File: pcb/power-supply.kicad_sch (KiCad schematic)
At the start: 6 parts, among them IC1 AP2112K-3.3TRG1

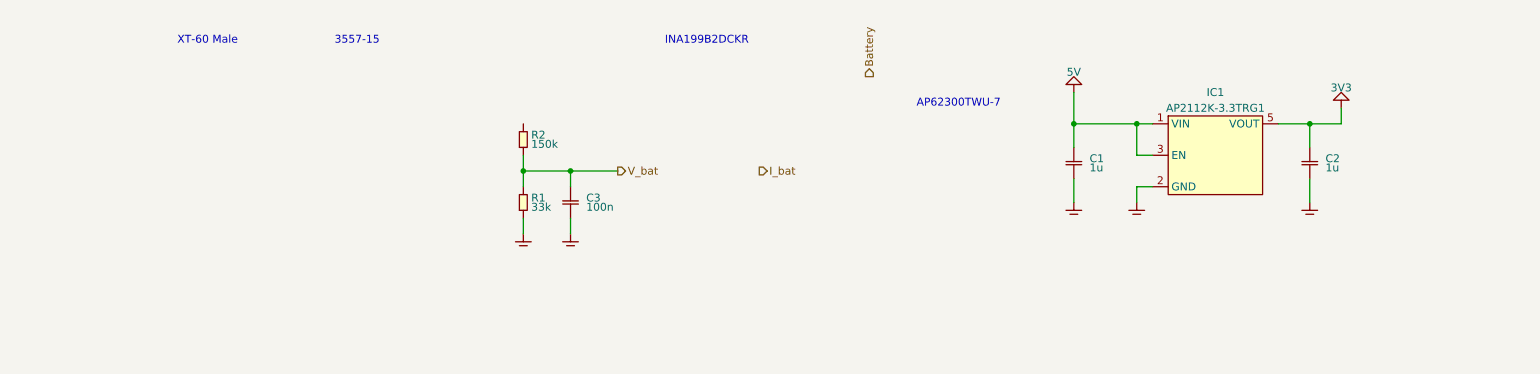
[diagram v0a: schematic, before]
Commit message: continued work on schematic
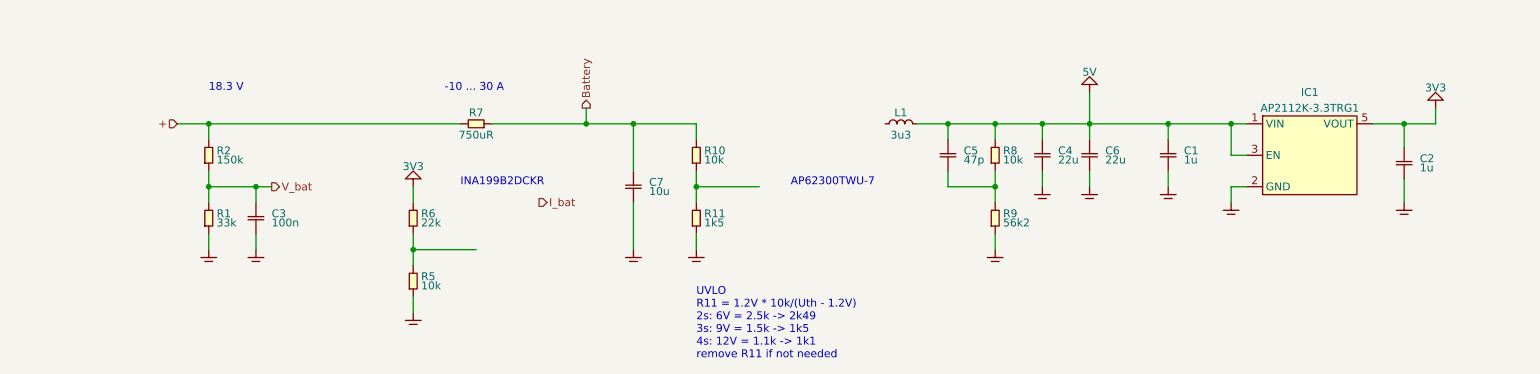
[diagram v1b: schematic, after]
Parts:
- added C4, C6: 22u, SMT:0603, symbol generic:C
- added C5: 47p, SMT:0603, symbol generic:C
- added C7: 10u, SMT:0603, symbol generic:C
- added L1: 3u3, symbol generic:L
- added R10, R5, R8: 10k, SMT:0603, symbol generic:R
- added R11: 1k5, SMT:0603, symbol generic:R
- added R6: 22k, SMT:0603, symbol generic:R
- added R7: 750uR, SMT:0603, symbol generic:R
- added R9: 56k2, SMT:0603, symbol generic:R
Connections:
- net 3V3: now also R6.2
- net Battery: now also C7.1, R10.2, R7.1
- net GND: now also C4.1, C4.2, C5.1, C6.1, C6.2, C7.2, L1.2, R11.1, R5.1, R8.2, R9.1
- net +: now reaches R2.2
- net +: now also R7.2
- new net: R10.1, R11.2
- new net: R5.2, R6.1
- new net: C5.2, R8.1, R9.2
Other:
- note added: "-10 ... 30 A"
- note added: "18.3 V"
- note added: "UVLO R11 = 1.2V * 10k/(Uth - 1.2V) 2s: 6V = 2.5k -> 2k49 3s: 9V = 1.5k -> 1k5 4s: 12V = 1.1k -> 1k1 remove R11 if not needed"
- note removed: "3557-15"
- note removed: "XT-60 Male"
- moved on the sheet: C1, C2, C3, IC1, R1, R2

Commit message: schematic mostly done
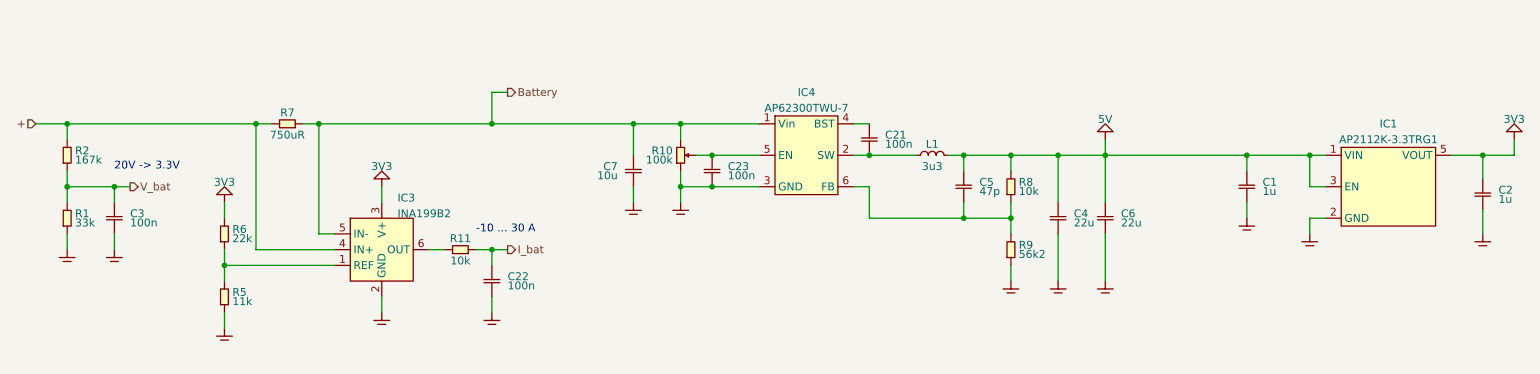
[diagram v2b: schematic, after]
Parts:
- removed R10: 10k, SMT:0603, symbol generic:R
- added C21, C22, C23: 100n, SMT:0603, symbol generic:C
- added IC3: INA199B2, symbol amplifiers:INA199B2
- added IC4: AP62300TWU-7, SOT:SOT-23-6, symbol Power:AP62300TWU-7
- added R10: 100k, symbol generic:Trimmer
- R11: value 1k5 -> 10k
- R2: value 150k -> 167k
- R5: value 10k -> 11k
- R7: footprint SMT:0603 -> (none)
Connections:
- net +: now also IC3.4 (IN+)
- net 3V3: now also IC3.3 (V+)
- net Battery: now also IC3.5 (IN-), IC4.1 (Vin), R10.3
- net GND: now also C22.2, C23.2, IC3.2 (GND), IC4.3 (GND), R10.1; no longer R11.1
- net I_bat: now also R11.1, C22.1
- net at R11.2: now also IC3.6 (OUT)
- net at R5.2, R6.1: now also IC3.1 (REF)
- net at C5.2, R8.1, R9.2: now also IC4.6 (FB)
- net at L1.1: now also C21.2, IC4.2 (SW)
- new net: C23.1, IC4.5 (EN), R10.2
- new net: C21.1, IC4.4 (BST)
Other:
- note added: "20V -> 3.3V"
- note removed: "18.3 V"
- note removed: "AP62300TWU-7"
- note removed: "INA199B2DCKR"
- note removed: "UVLO R11 = 1.2V * 10k/(Uth - 1.2V) 2s: 6V = 2.5k -> 2k49 3s: 9V = 1.5k -> 1k5 4s: 12V = 1.1k -> 1k1 remove R11 if not needed"
- title: (none) -> CAN bus to RC servo adapter
- moved on the sheet: C1, C2, C3, C4, C5, C6, C7, IC1, L1, R1, R2, R5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
